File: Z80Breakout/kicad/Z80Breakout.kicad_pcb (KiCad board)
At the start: 2 copper layers, 64.5 x 62 mm, 5 parts, among them J1 Pin1:20, J2 Pin21:40, J3 Host Z80, U1 Z80CPU

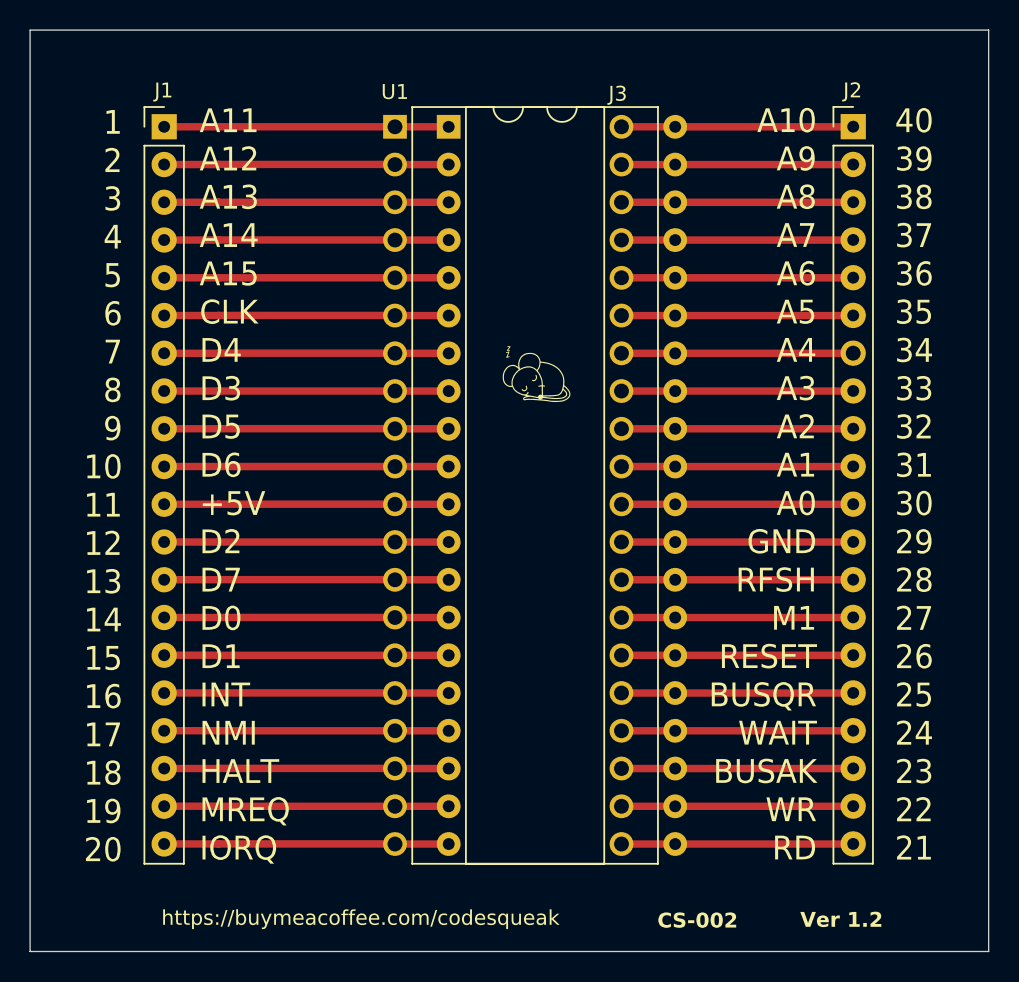
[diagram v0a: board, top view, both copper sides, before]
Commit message: Z80 Breakout
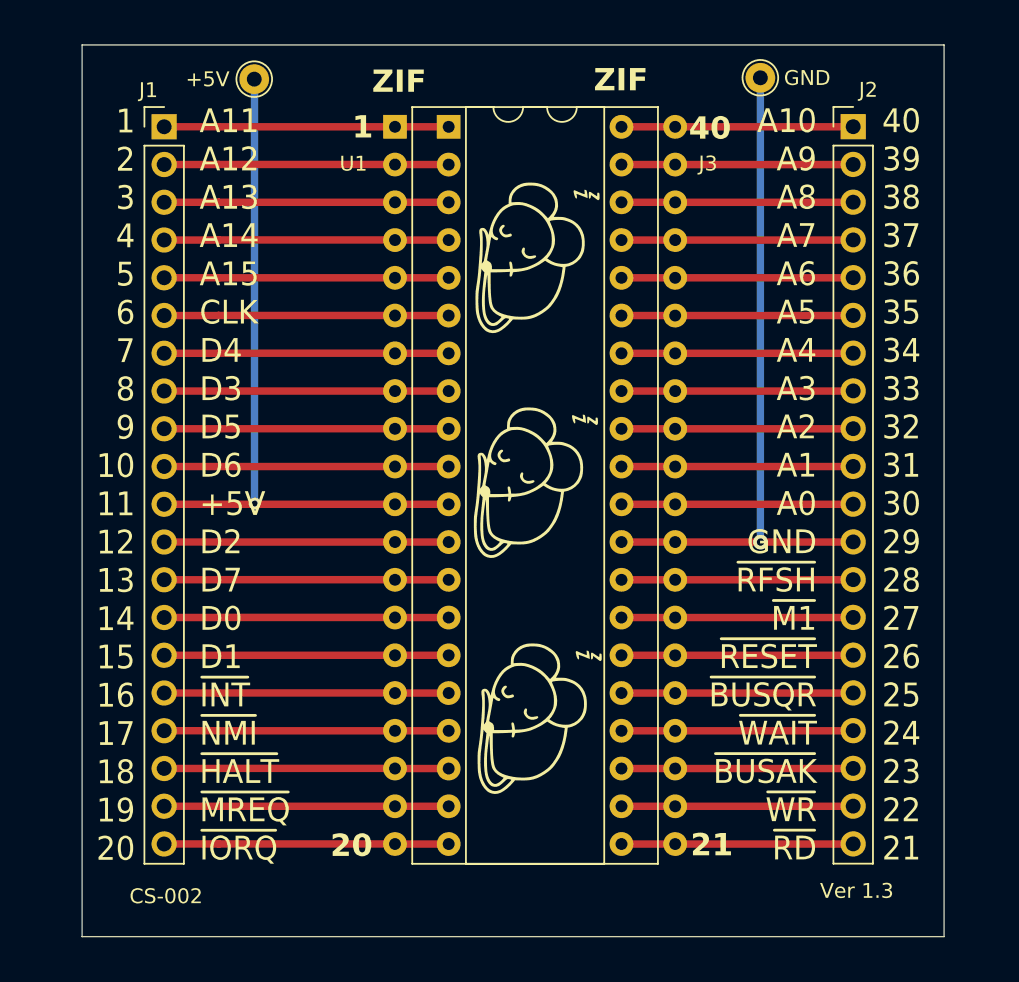
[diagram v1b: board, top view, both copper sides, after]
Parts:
- removed the G1 at (140.4, 73.3)
- added G1: LOGO, 80bus:sleepymouse_very_very_small, F.Cu at (140.7, 96.4)
- added G1: LOGO, 80bus:sleepymouse_very_very_small, F.Cu at (140.6, 65.4)
- added G1: LOGO, 80bus:sleepymouse_very_very_small, F.Cu at (140.5, 80.5)
- added TP1: GND, TestPoint:TestPoint_THTPad_D2.0mm_Drill1.0mm, F.Cu at (155.6, 53.2)
- added TP2: +5V, TestPoint:TestPoint_THTPad_D2.0mm_Drill1.0mm, F.Cu at (121.6, 53.3)
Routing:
- net GND: track 15.6 -> 46.8 mm, vias 0 -> 1
- net VCC: track 19.1 -> 47.2 mm, vias 0 -> 1
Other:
- board size 64.5 x 62 mm -> 58 x 60 mm
- board text added: "1"
- board text added: "20"
- board text added: "21"
- board text added: "40"
- board text added: "A10 A9 A8 A7 A6 A5 A4 A3 A2 A1 A0 GND ~{RFSH} ~{M1} ~{RESET} ~{BUSQR} ~{WAIT} ~{BUSAK} ~{WR} ~{RD}"
- board text added: "A11 A12 A13 A14 A15 CLK D4 D3 D5 D6 +5V D2 D7 D0 D1 ~{INT} ~{NMI} ~{HALT} ~{MREQ} ~{IORQ}"
- board text added: "Ver 1.3"
- board text added: "ZIF"
- board text added: "abd18f6a-026c-42df-9f07-f37d9ccea511"
- board text removed: "A10 A9 A8 A7 A6 A5 A4 A3 A2 A1 A0 GND RFSH M1 RESET BUSQR WAIT BUSAK WR RD"
- board text removed: "A11 A12 A13 A14 A15 CLK D4 D3 D5 D6 +5V D2 D7 D0 D1 INT NMI HALT MREQ IORQ"
- board text removed: "Ver 1.2"
- board text removed: "b0efcf87-67be-433f-902f-6073ec17ba45"
- board text removed: "https://buymeacoffee.com/codesqueak"
